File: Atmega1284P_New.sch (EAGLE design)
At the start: 49 parts, among them U2 ATMEGA1284P-AU, U3 ESP-WROOM-32

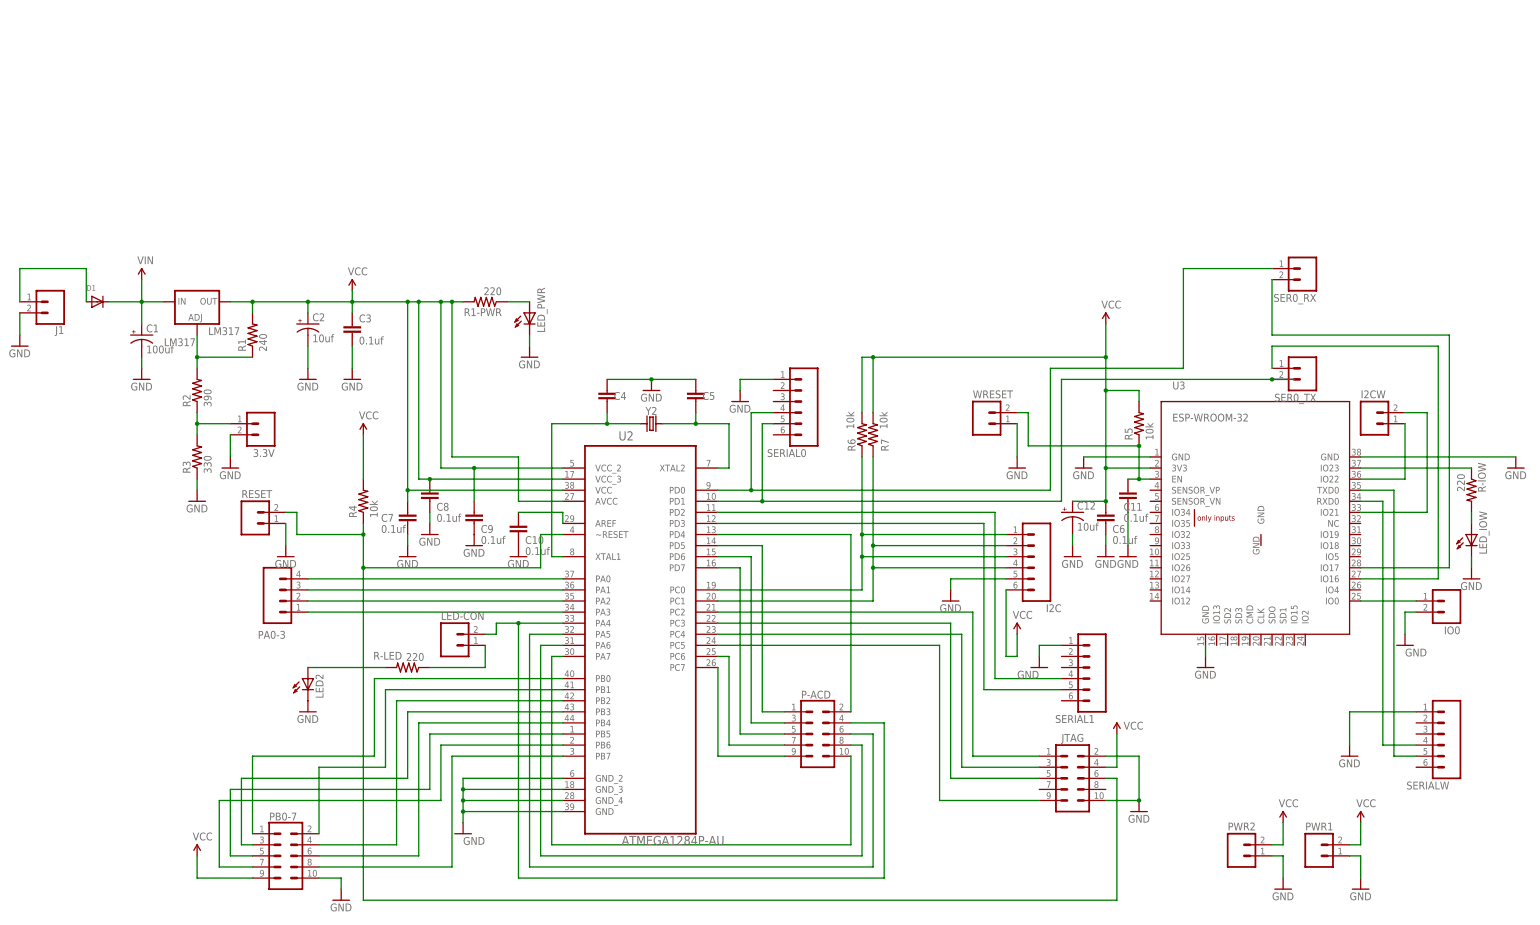
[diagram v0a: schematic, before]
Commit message: GOOD_Working_Copy
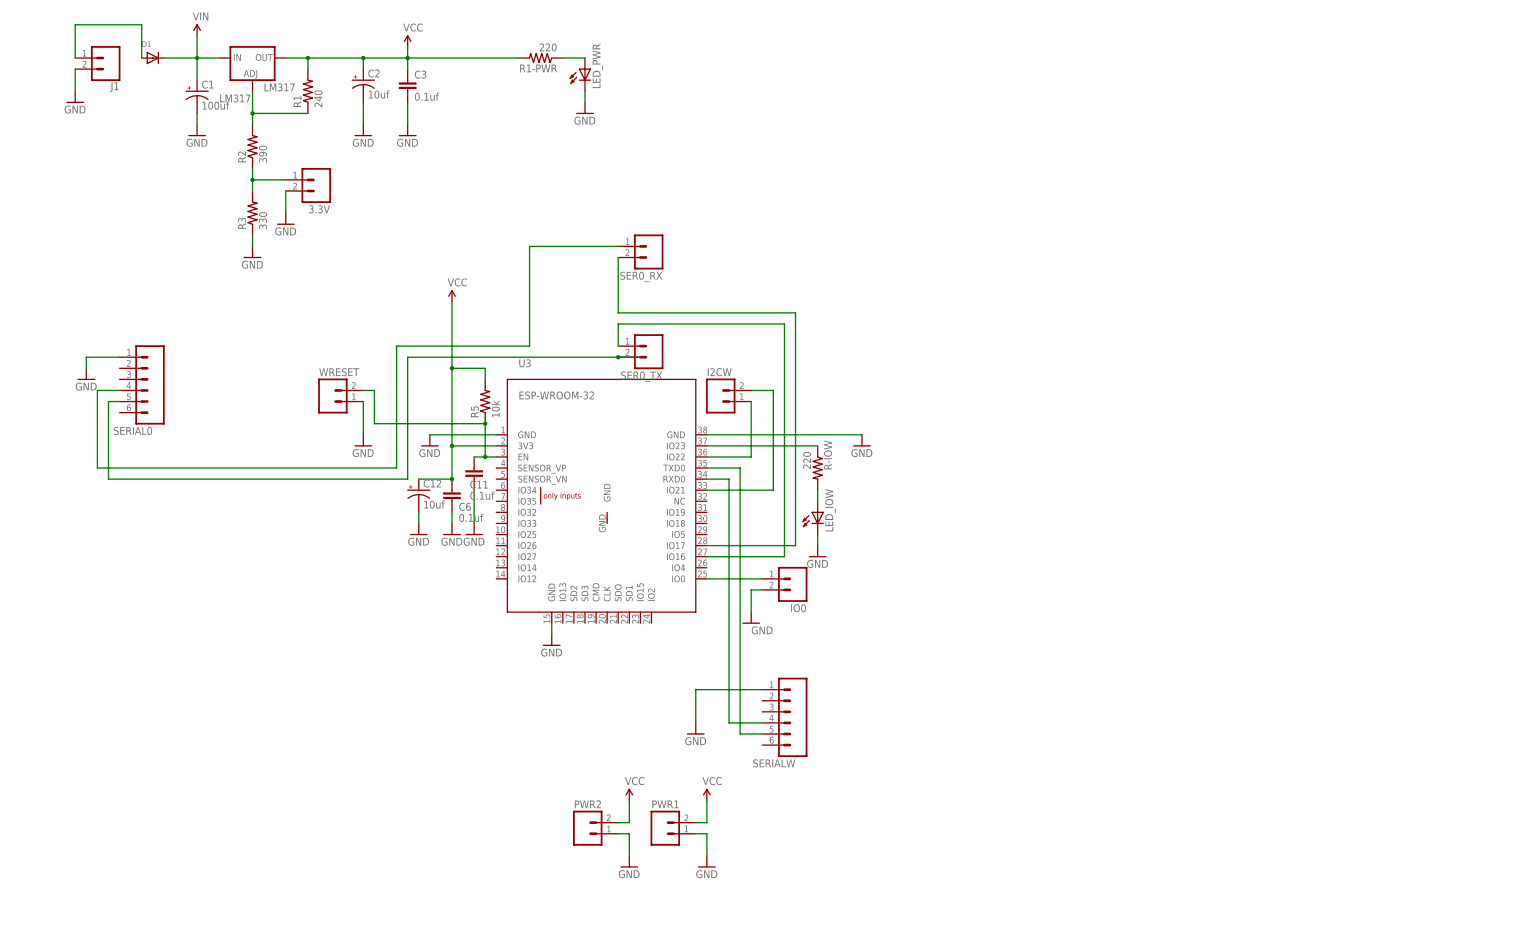
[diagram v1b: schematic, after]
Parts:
- removed C10, C7, C8, C9: 0.1uf, SparkFun-Passives:CAP0805
- removed C4, C5: (no value), SparkFun-Passives:CAP0805
- removed I2C, SERIAL1: (no value), SparkFun-Connectors:M06SILK_FEMALE_PTH
- removed JTAG: (no value), SparkFun-Connectors:M05X2PTH
- removed LED-CON, RESET: (no value), SparkFun-Connectors:M02PTH
- removed LED2: (no value), adafruit:LEDCHIPLED_0805
- removed P-ACD, PB0-7: (no value), SparkFun-Connectors:CONN_05X2PTH
- removed PA0-3: (no value), SparkFun-Connectors:M04PTH
- removed R-LED: 220, resistor:R-US_R0805
- removed R4, R6, R7: 10k, resistor:R-US_R0805
- removed U2: ATMEGA1284P-AU, Atmel_By_element14_Batch_1-00:ATMEGA1284P-AU
- removed Y2: (no value), SparkFun-Clocks:CRYSTALSMD-5X3.2-2PAD
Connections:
- removed net N$10: JTAG.1, U2.PC2
- removed net N$11: JTAG.5, U2.PC3
- removed net N$12: JTAG.9, U2.PC5
- removed net N$14: C4.2, U2.XTAL1, Y2.1
- removed net N$15: PA0-3.4, U2.PA0
- removed net N$16: PA0-3.3, U2.PA1
- removed net N$17: PA0-3.2, U2.PA2
- removed net N$18: PA0-3.1, U2.PA3
- removed net N$19: LED-CON.1, R-LED.1
- removed net N$2: PB0-7.3, U2.PB3
- removed net N$20: LED2.A, R-LED.2
- removed net N$21: I2C.1, I2C.3, R6.1, U2.PC0
- removed net N$22: I2C.2, I2C.4, R7.1, U2.PC1
- removed net N$23: PB0-7.1, U2.PB0
- removed net N$24: PB0-7.2, U2.PB1
- removed net N$25: PB0-7.4, U2.PB2
- removed net N$26: PB0-7.8, U2.PB7
- removed net N$27: PB0-7.5, U2.PB5
- removed net N$28: PB0-7.6, U2.PB4
- removed net N$29: PB0-7.7, U2.PB6
- removed net N$30: JTAG.6, R4.1, RESET.2, U2.~RESET
- removed net N$31: P-ACD.9, U2.PC7
- removed net N$32: P-ACD.7, U2.PC6
- removed net N$33: P-ACD.5, U2.PD7
- removed net N$34: P-ACD.3, U2.PD6
- removed net N$35: P-ACD.1, U2.PD5
- removed net N$36: P-ACD.2, U2.PD4
- removed net N$37: P-ACD.10, U2.PA7
- removed net N$38: P-ACD.8, U2.PA6
- removed net N$39: P-ACD.6, U2.PA5
- removed net N$4: C10.1, U2.AREF
- removed net N$40: LED-CON.2, P-ACD.4, U2.PA4
- removed net N$6: C5.2, U2.XTAL2, Y2.2
- removed net N$7: SERIAL1.4, U2.PD2
- removed net N$8: SERIAL1.5, U2.PD3
- removed net N$9: JTAG.3, U2.PC4
- net GND: no longer C10.2, C4.1, C5.1, C7.2, C8.2, C9.2, I2C.5, JTAG.10, JTAG.2, LED2.C, PB0-7.10, RESET.1, SERIAL1.1, U2.GND, U2.GND_2, U2.GND_3, U2.GND_4
- net N$3: no longer U2.PD0
- net N$5: no longer U2.PD1
- net VCC: no longer C7.1, C8.1, C9.1, I2C.6, JTAG.4, PB0-7.9, R4.2, R6.2, R7.2, U2.AVCC, U2.VCC, U2.VCC_2, U2.VCC_3
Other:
- moved on the sheet: 3.3V, C1, C11, C12, C2, C3, C6, D1, I2CW, IO0, J1, LED_IOW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
